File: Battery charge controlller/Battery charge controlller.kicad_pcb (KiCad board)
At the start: 2 copper layers, 50 parts, among them J1 14V, J2 Conn_01x03, Q1 Si7336ADP, Q2 Si7336ADP, Q3 2N7002, U1 BQ24650

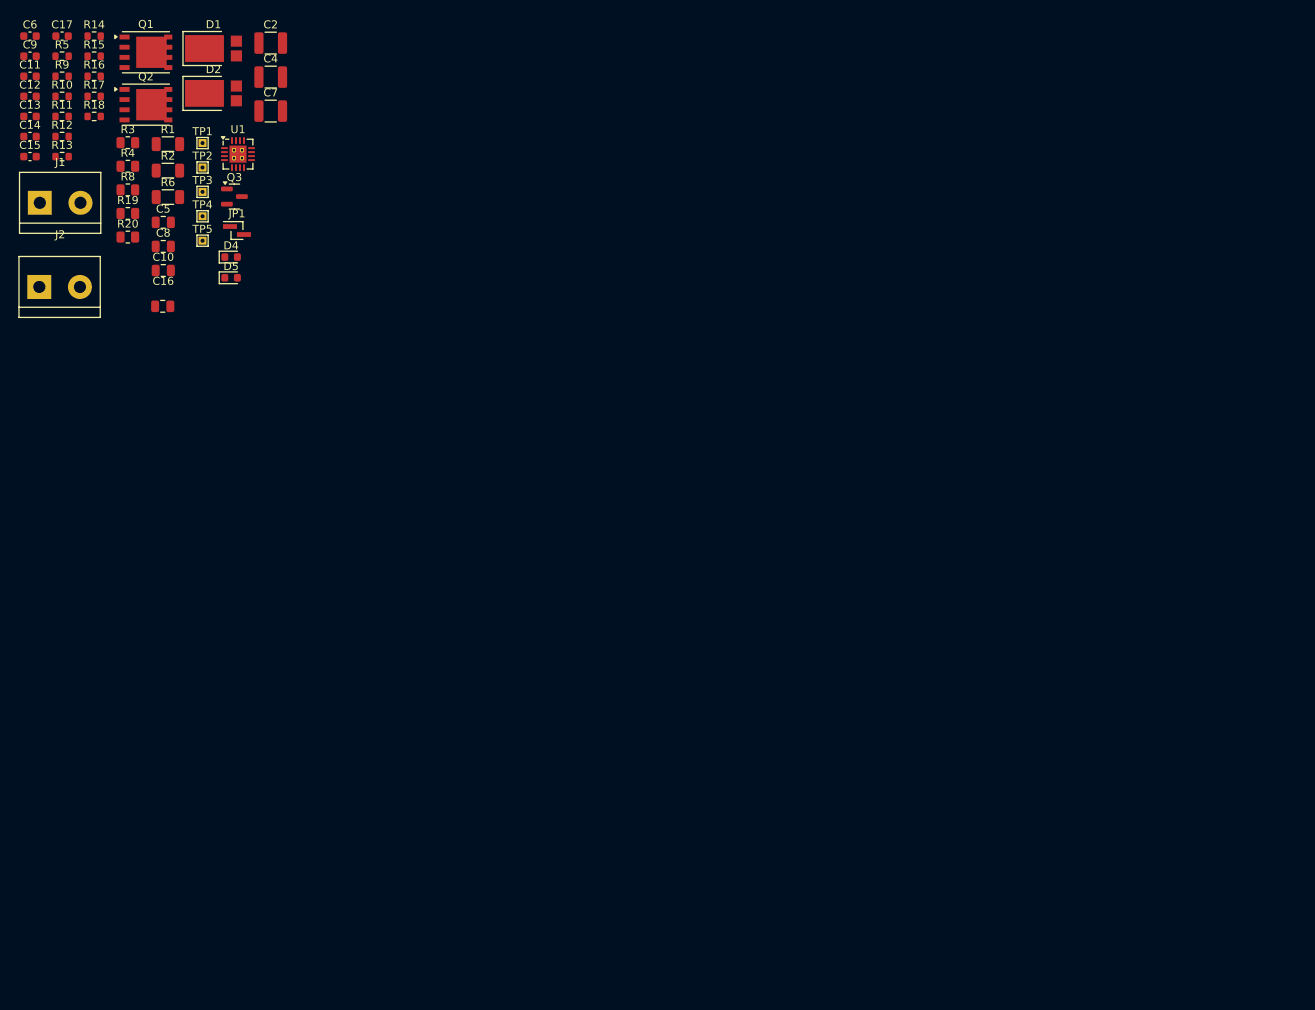
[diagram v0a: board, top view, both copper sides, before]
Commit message: EPS version 1
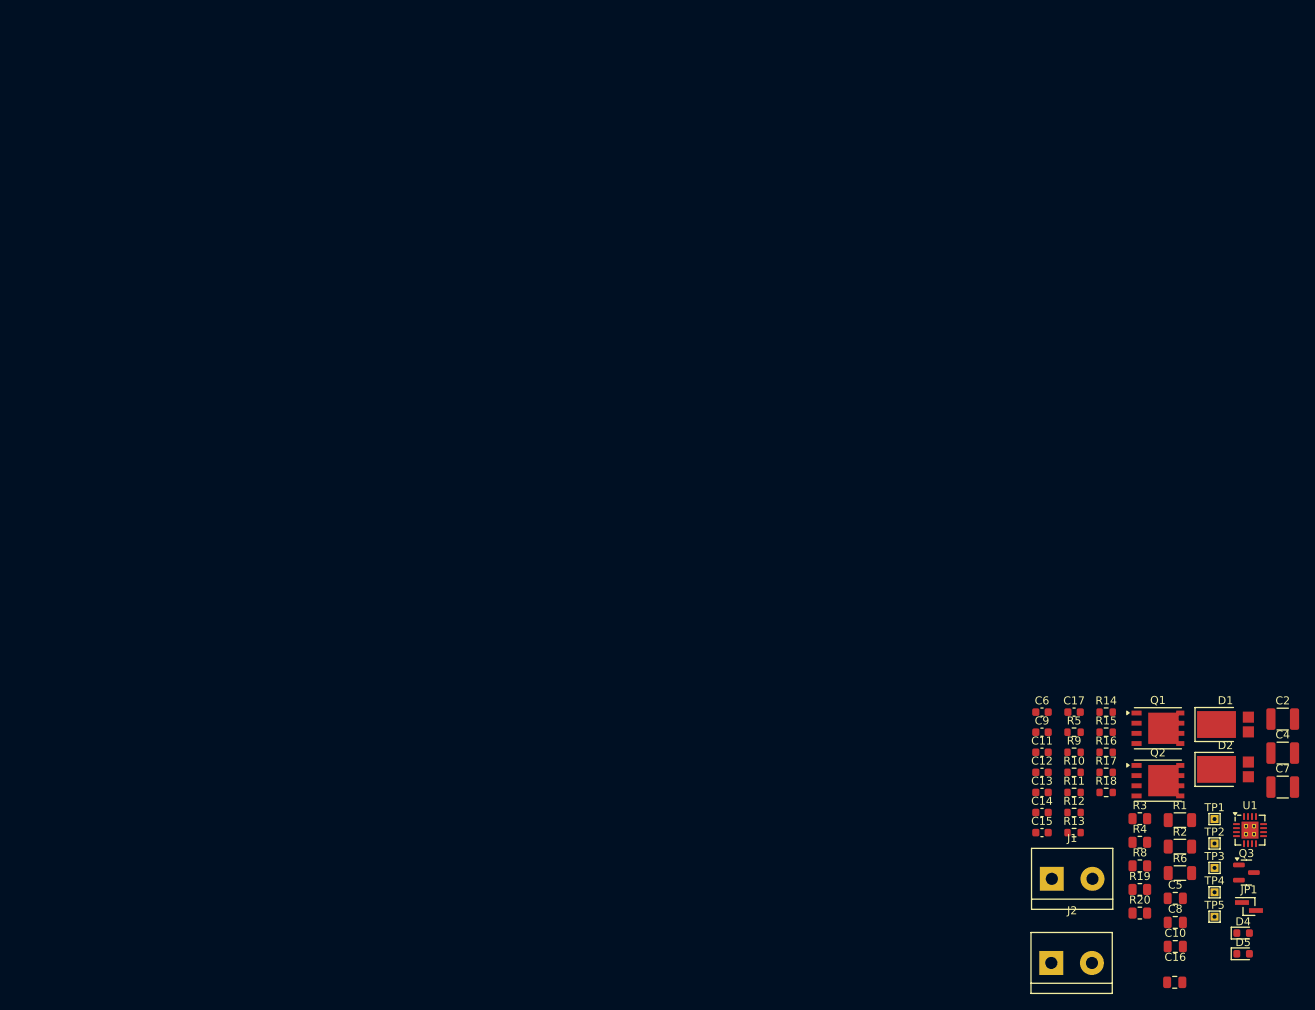
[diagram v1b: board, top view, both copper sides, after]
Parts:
- moved C17 152.1 mm to (132.1, 83.8)
- moved J1 152.1 mm to (129.3, 104.6)
- moved J2 152.1 mm to (129.2, 115.1)
- moved R10 152.1 mm to (132.1, 91.3)
- moved R11 152.1 mm to (132.1, 93.8)
- moved R12 152.1 mm to (132.1, 96.3)
- moved R13 152.1 mm to (132.1, 98.8)
- moved R19 152.1 mm to (140.3, 106.0)
- moved R20 152.1 mm to (140.3, 108.9)
- moved R3 152.1 mm to (140.3, 97.1)
- moved R4 152.1 mm to (140.3, 100.1)
- moved R5 152.1 mm to (132.1, 86.3)
- moved R8 152.1 mm to (140.3, 103.0)
- moved R9 152.1 mm to (132.1, 88.8)
- moved TP1 152.1 mm to (149.6, 97.2)
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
